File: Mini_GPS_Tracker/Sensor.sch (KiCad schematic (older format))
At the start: 13 parts, among them U2 MS5611-01BA, U7 LSM9DS1

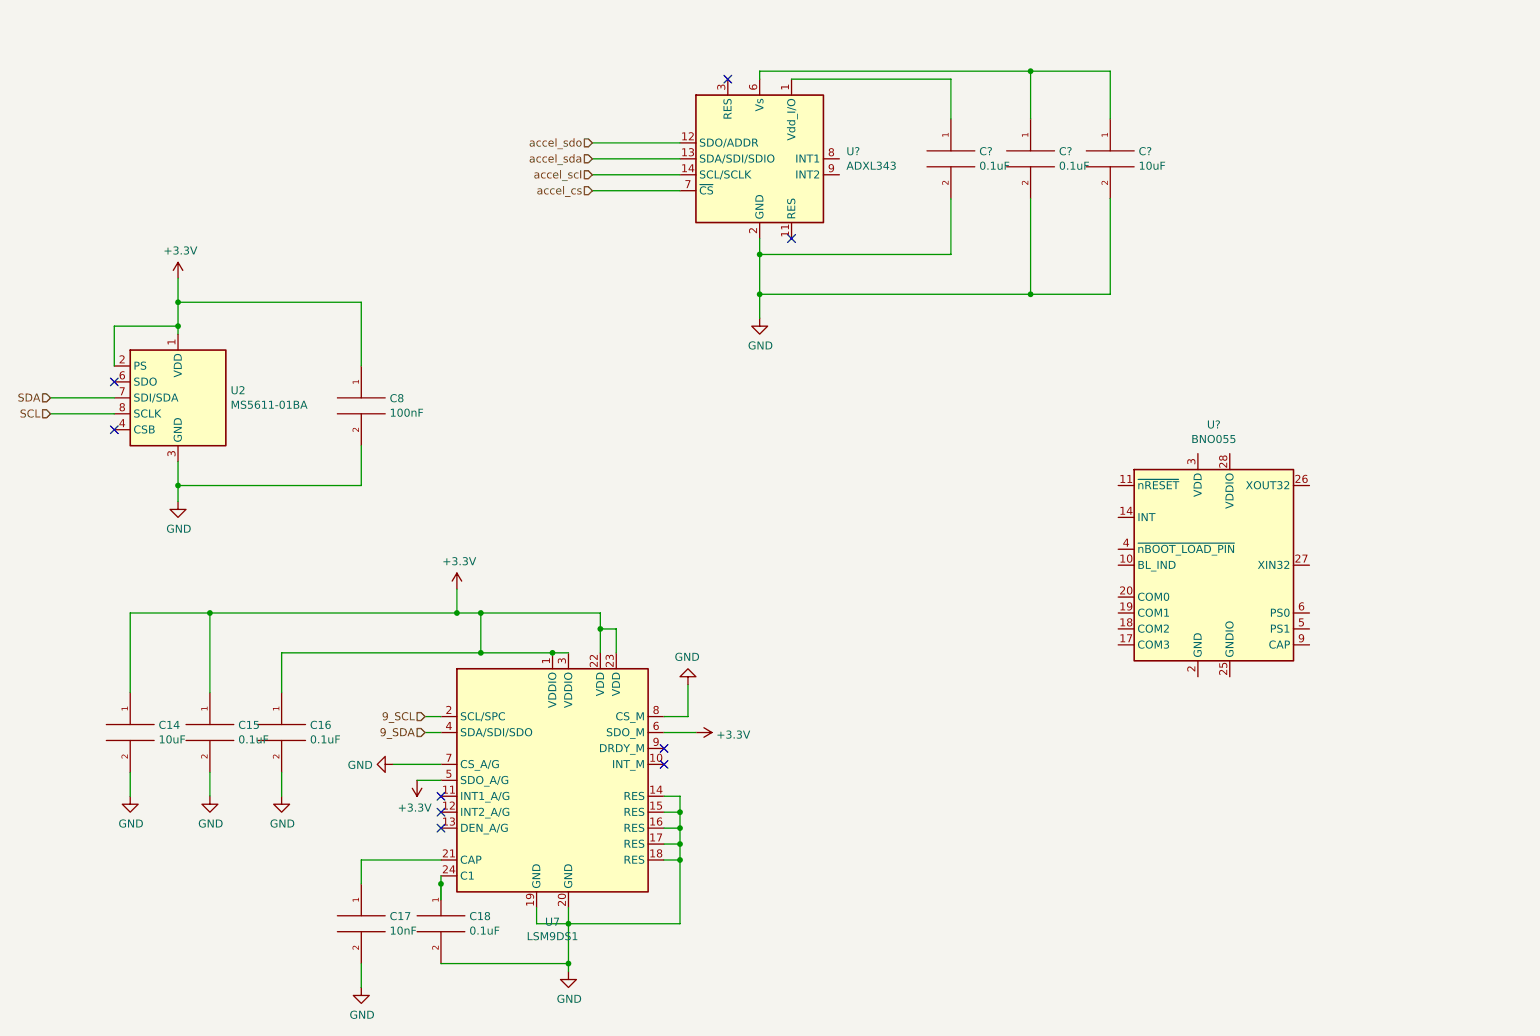
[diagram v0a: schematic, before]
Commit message: Add files via upload
Updates schematics
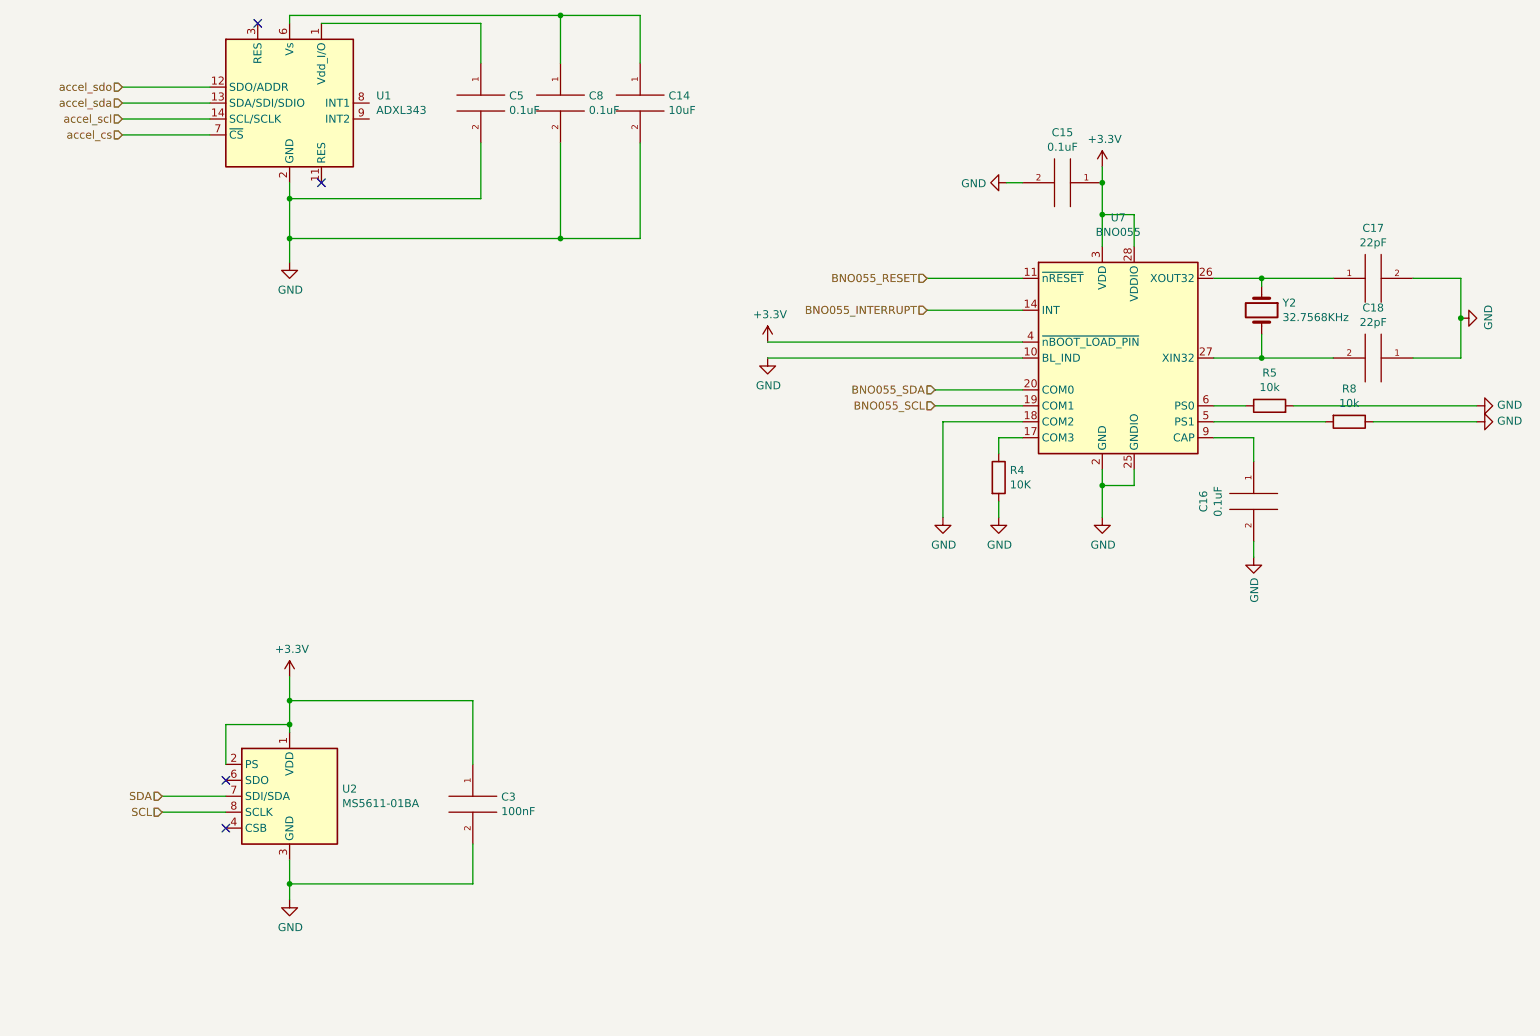
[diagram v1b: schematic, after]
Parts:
- removed C14: 10uF, Capacitor_SMD:C_0805_2012Metric_Pad1.15x1.40mm_HandSolder, symbol pspice:CAP
- removed U7: LSM9DS1, Package_LGA:LGA-24L_3x3.5mm_P0.43mm, symbol Sensor_Motion:LSM9DS1
- added R4: 10K, Resistor_SMD:R_0805_2012Metric_Pad1.15x1.40mm_HandSolder, symbol Device:R
- added R5, R8: 10k, Resistor_SMD:R_0805_2012Metric_Pad1.15x1.40mm_HandSolder, symbol Device:R
- added Y2: 32.7568KHz, Crystal:Crystal_SMD_2012-2Pin_2.0x1.2mm_HandSoldering, symbol Device:Crystal
- C14, C5, C8: renamed from C?; footprint (none) -> Capacitor_SMD:C_0805_2012Metric_Pad1.15x1.40mm_HandSolder
- C17: value 10nF -> 22pF
- C18: value 0.1uF -> 22pF
- gave numbers to parts that had none: 2
- renumbered C8 to C3
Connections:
- net +3V3: now also U7.28 (VDDIO), U7.3 (VDD), U7.4 (~nBOOT_LOAD_PIN); no longer C16.1
- net GND: now also C18.1, U7.10 (BL_IND), U7.15 (GNDIO), U7.16 (GNDIO), U7.18 (COM2), U7.2 (GND), U7.25 (GNDIO), R4.2, R5.2, R8.1; no longer C18.2
- net at C17.1: now also U7.26 (XOUT32), Y2.1
- net BNO055_RESET: now reaches U7.11 (~nRESET)
- net BNO055_INTERRUPT: now reaches U7.14 (INT)
- net at U7.17 (COM3): now also R4.1
- net BNO055_SCL: now reaches U7.19 (COM1)
- net BNO055_SDA: now reaches U7.20 (COM0)
- net at U7.27 (XIN32): now also C18.2, Y2.2
- net at U7.5 (PS1): now also R8.2
- net at U7.6 (PS0): now also R5.1
- net at U7.9 (CAP): now also C16.1
- no-connect marks 9 -> 4
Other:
- moved on the sheet: C14, C3, C5, C8, U1, U2, U7
